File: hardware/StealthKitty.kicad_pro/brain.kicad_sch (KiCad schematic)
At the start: 26 parts, among them J401 Conn_ST_STDC14, SW401 SW_Push, SW402 SW_Push, U401 STM32G431CBU6, Y401 Crystal_GND24_Small

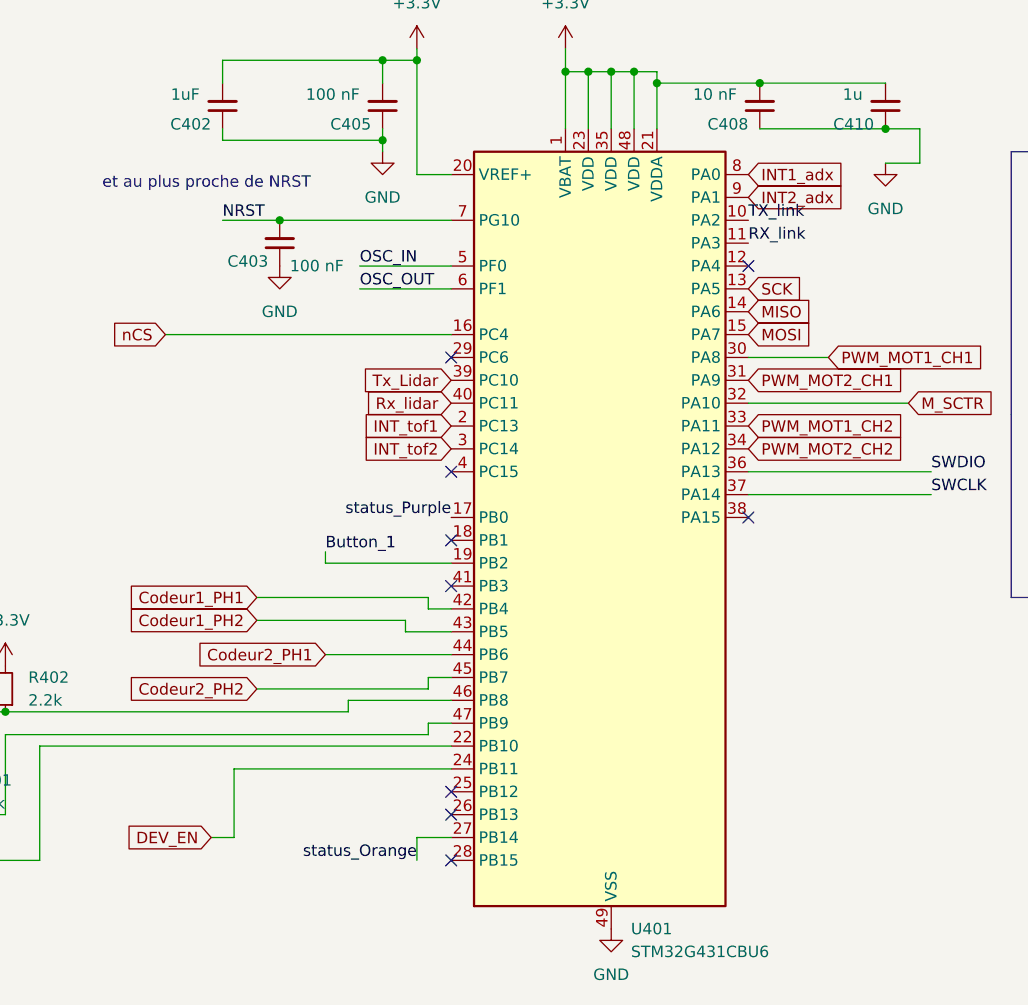
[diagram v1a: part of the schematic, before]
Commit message: Dernier Modif 08/10/2024
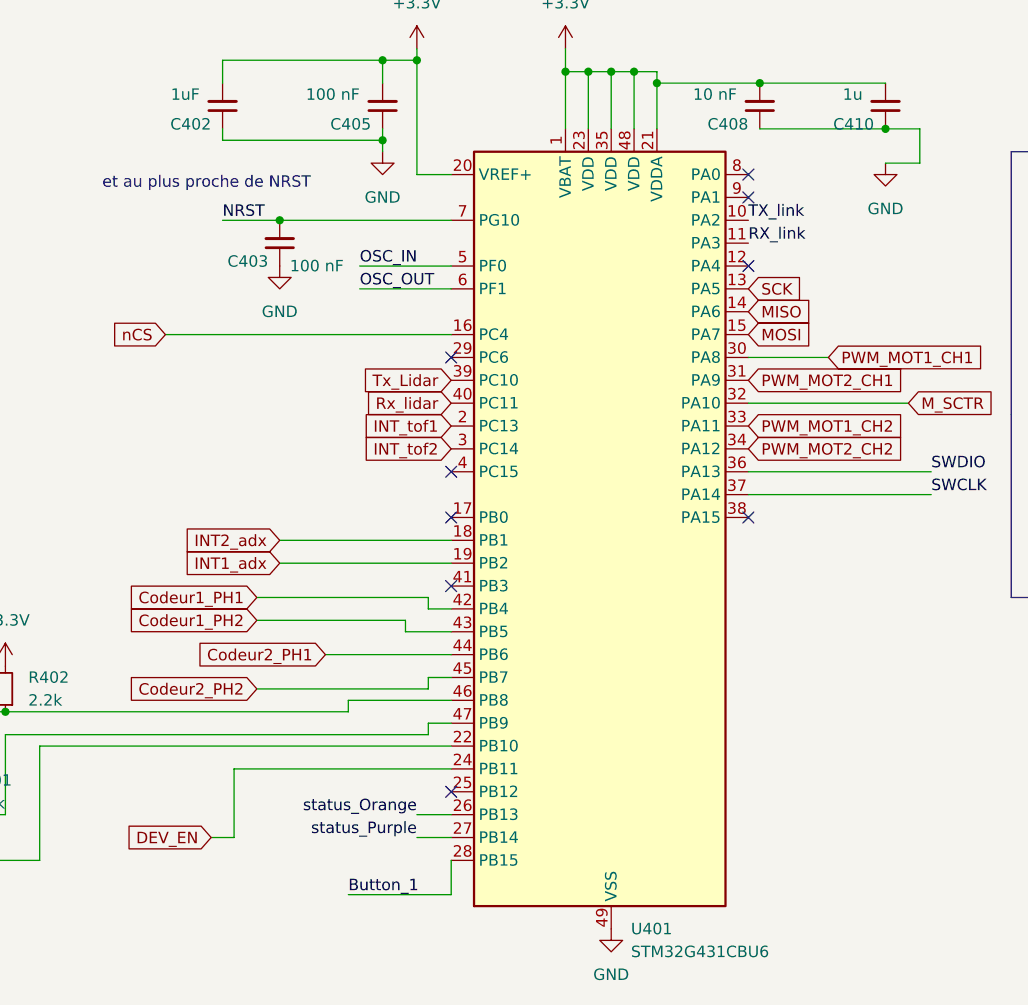
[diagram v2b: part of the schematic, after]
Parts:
- C401, C403, C404, C405, C406, C408, C409, C411: footprint Capacitor_SMD:C_0402_1005Metric_Pad0.74x0.62mm_HandSolder -> Capacitor_SMD:C_0402_1005Metric
- C402, C407, C410: footprint Capacitor_SMD:C_0603_1608Metric_Pad1.08x0.95mm_HandSolder -> Capacitor_SMD:C_0402_1005Metric
- R401, R402, R403, R404: footprint Resistor_SMD:R_0603_1608Metric_Pad0.98x0.95mm_HandSolder -> Resistor_SMD:R_0402_1005Metric
- SW401, SW402: footprint Button_Switch_SMD:SW_SPST_B3U-1000P -> Button_Switch_SMD:SW_Push_1P1T_NO_6x6mm_H9.5mm
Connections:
- net Button_1: now also U401.28 (PB15); no longer U401.19 (PB2)
- net INT1_adx: now also U401.19 (PB2); no longer U401.8 (PA0)
- net INT2_adx: now also U401.18 (PB1); no longer U401.9 (PA1)
- net status_Orange: now also U401.26 (PB13); no longer U401.27 (PB14)
- net status_Purple: now also U401.27 (PB14); no longer U401.17 (PB0)
